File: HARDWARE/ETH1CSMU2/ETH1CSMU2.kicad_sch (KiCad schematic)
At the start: 0 parts

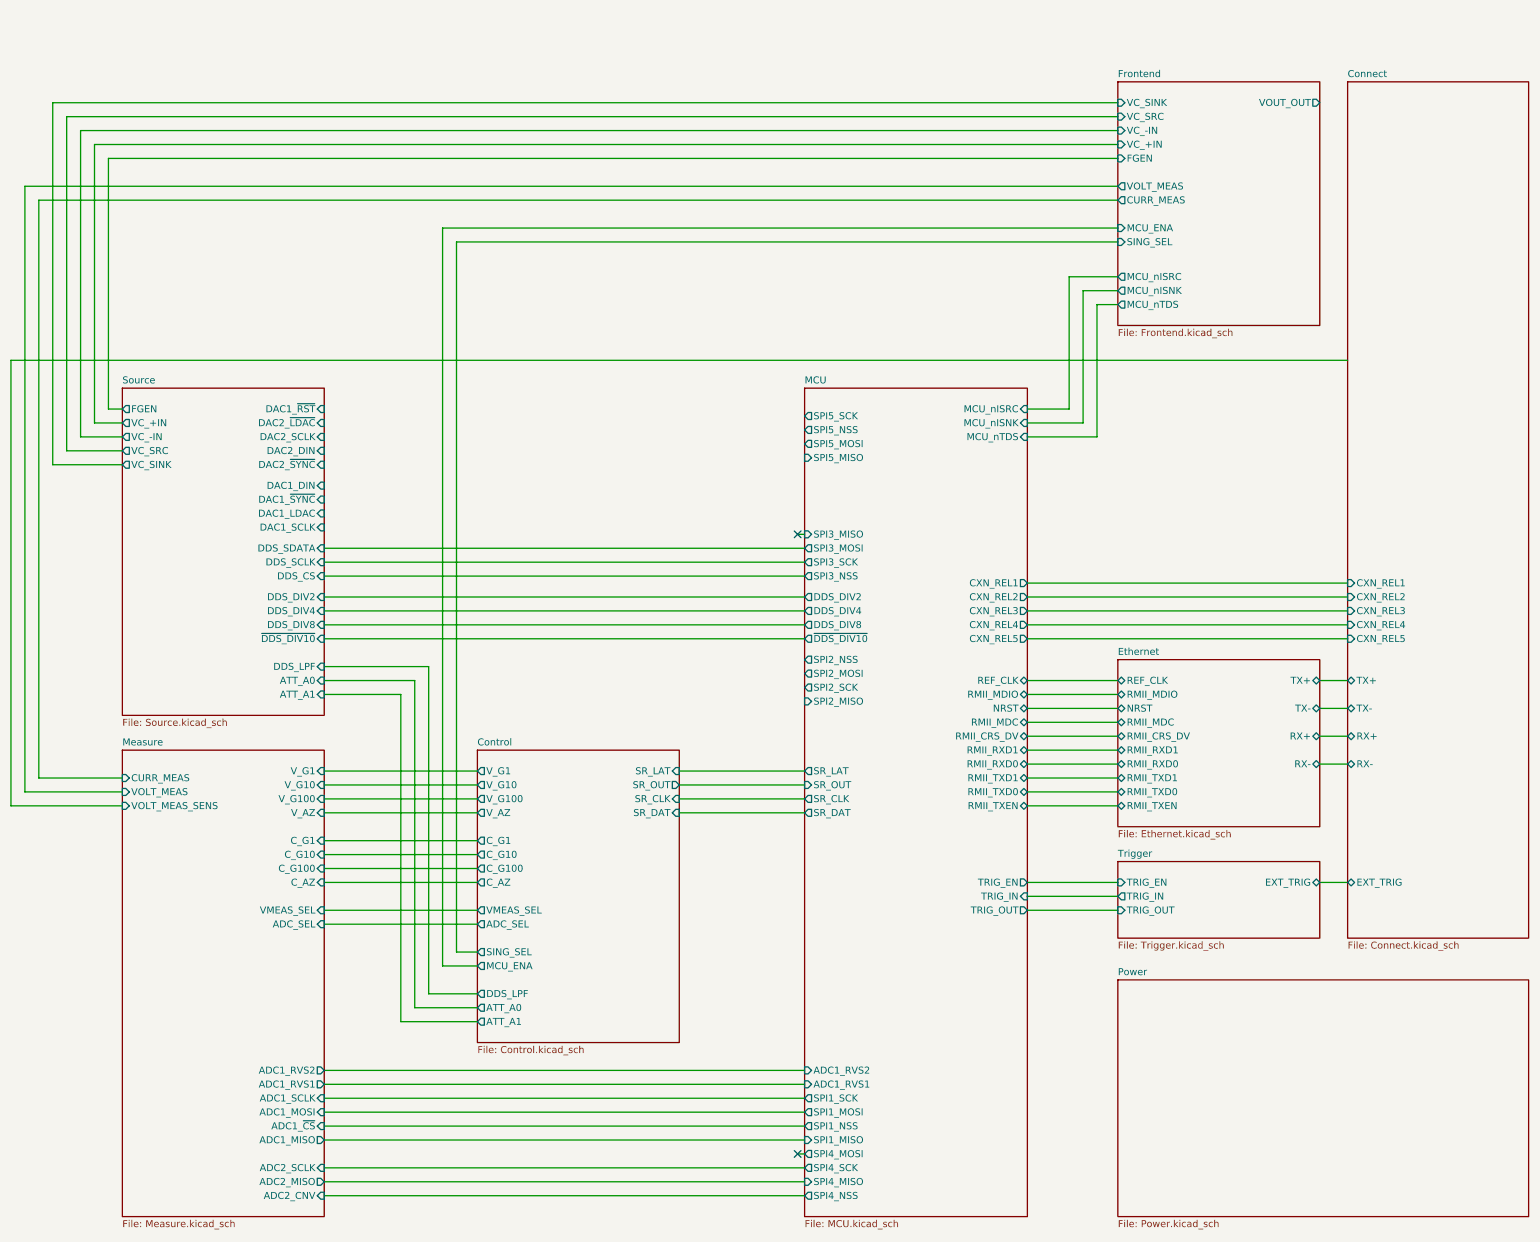
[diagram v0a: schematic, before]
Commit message: CRC check
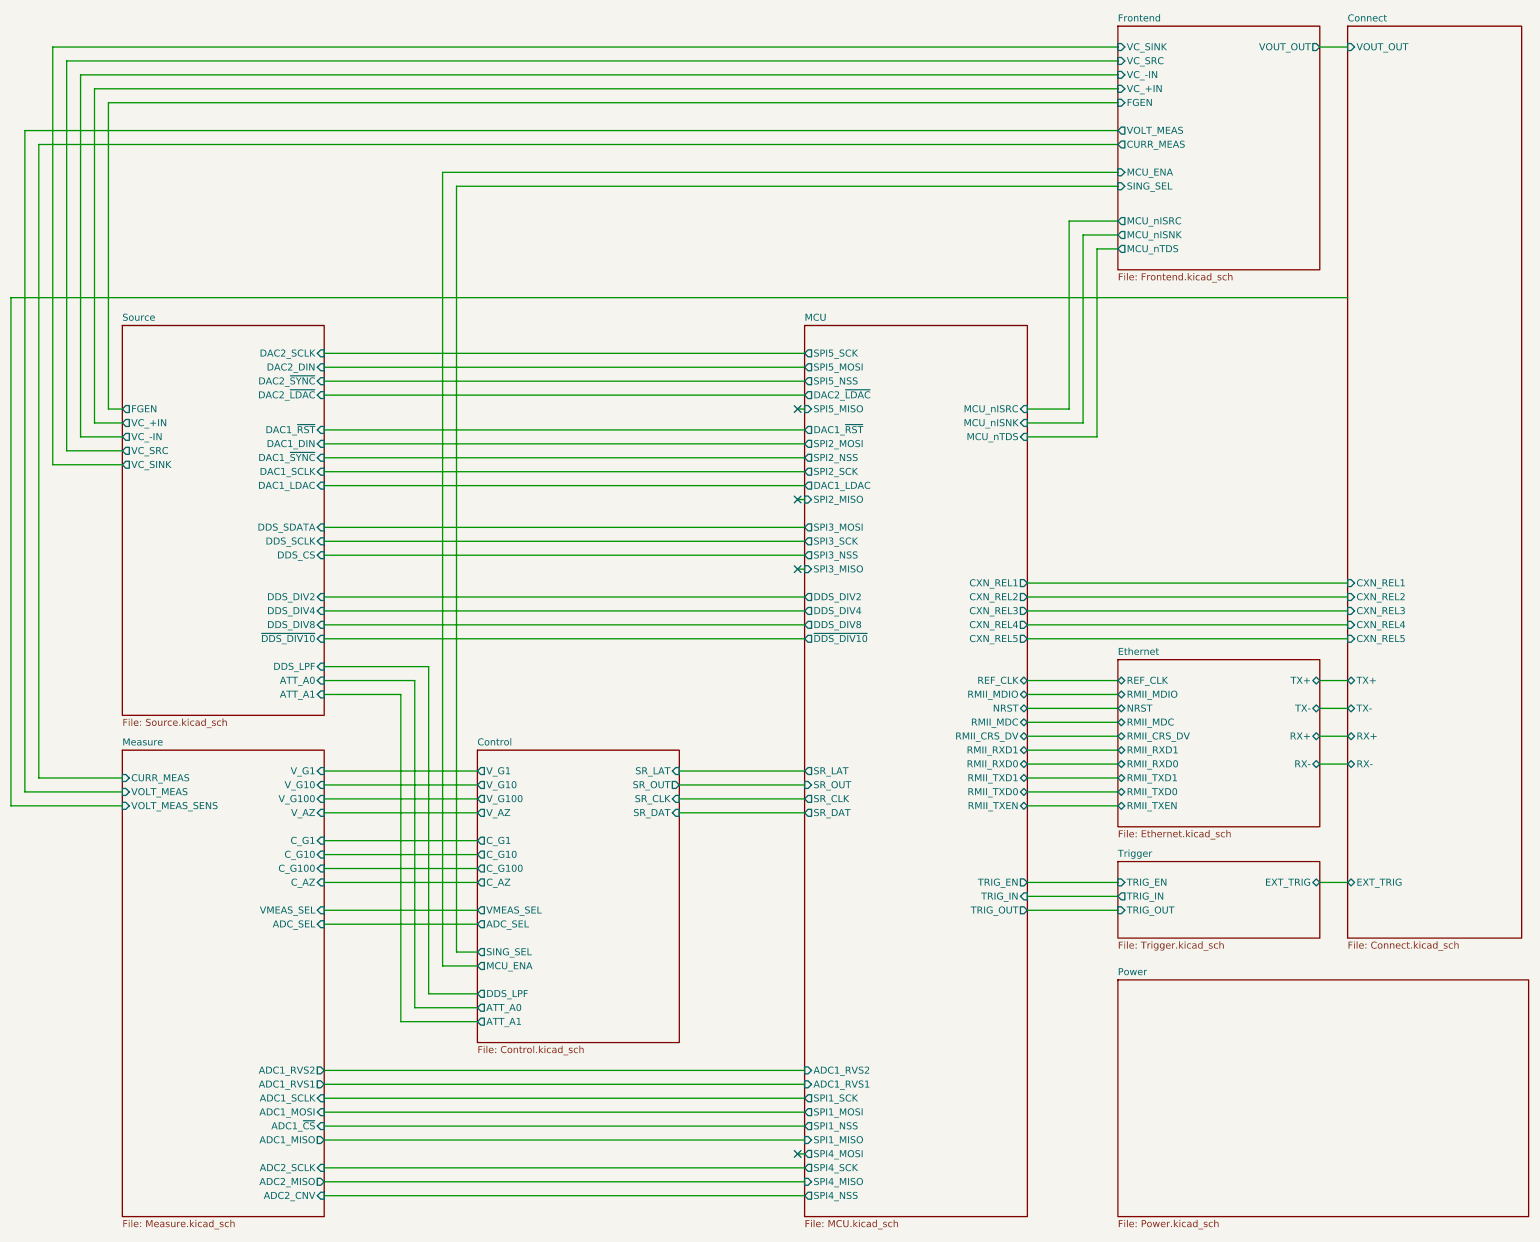
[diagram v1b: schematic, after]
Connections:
- no-connect marks 2 -> 4
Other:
- sheet Connect ports: added VOUT_OUT; removed none
- sheet MCU ports: added DAC1_LDAC, DAC1_~{RST}, DAC2_~{LDAC}; removed none
